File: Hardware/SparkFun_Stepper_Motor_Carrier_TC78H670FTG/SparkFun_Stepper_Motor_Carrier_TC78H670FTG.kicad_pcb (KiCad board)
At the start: 4 copper layers, 15.2 x 20.3 mm, 34 parts, among them J1 Conn_01x08, J2 Conn_01x08

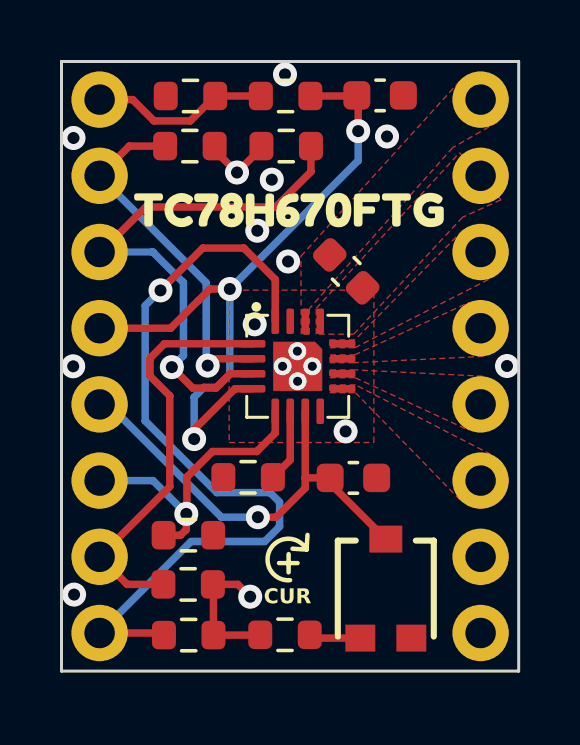
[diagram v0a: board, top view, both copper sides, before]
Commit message: version in bottom copper
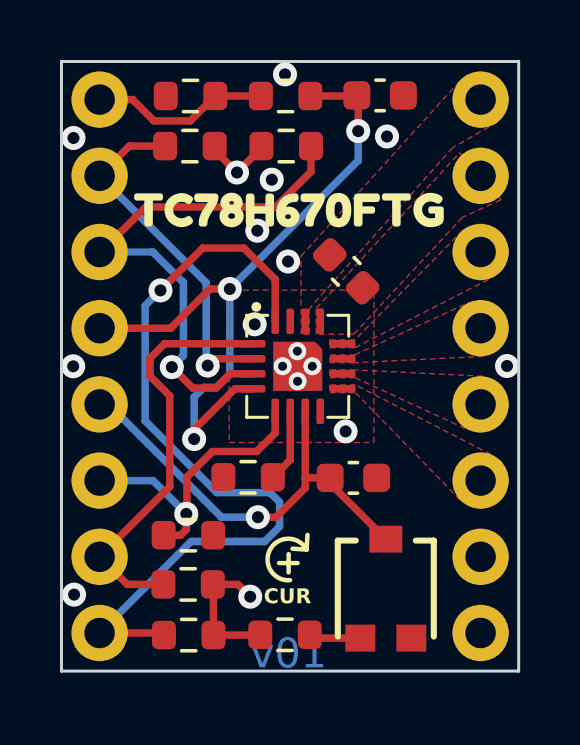
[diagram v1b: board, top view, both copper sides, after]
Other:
- board text added: "v01"
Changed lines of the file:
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@@
   (setup
     (stackup
-      (layer "F.SilkS" (type "Top Silk Screen"))
+      (layer "F.SilkS" (type "Top Silk Screen") (color "White"))
       (layer "F.Paste" (type "Top Solder Paste"))
-      (layer "F.Mask" (type "Top Solder Mask") (thickness 0.01))
+      (layer "F.Mask" (type "Top Solder Mask") (color "Red") (thickness 0.01))
       (layer "F.Cu" (type "copper") (thickness 0.035))
       (layer "dielectric 1" (type "prepreg") (thickness 0.1) (material "FR4") (epsilon_r 4.5) (loss_tangent 0.02))
@@
       (layer "dielectric 3" (type "prepreg") (thickness 0.1) (material "FR4") (epsilon_r 4.5) (loss_tangent 0.02))
       (layer "B.Cu" (type "copper") (thickness 0.035))
-      (layer "B.Mask" (type "Bottom Solder Mask") (thickness 0.01))
+      (layer "B.Mask" (type "Bottom Solder Mask") (color "Red") (thickness 0.01))
       (layer "B.Paste" (type "Bottom Solder Paste"))
-      (layer "B.SilkS" (type "Bottom Silk Screen"))
+      (layer "B.SilkS" (type "Bottom Silk Screen") (color "White"))
       (copper_finish "None")
       (dielectric_constraints no)
@@
   (gr_rect (start 134.62 93.98) (end 149.86 114.3)
     (stroke (width 0.1) (type default)) (fill none) (layer "Edge.Cuts"))
+  (gr_text "v01" (at 140.91 114.3) (layer "B.Cu")
+    (effects (font (size 1 1) (thickness 0.15)) (justify left bottom))
+  )
   (gr_text "CUR" (at 141.36 112.1) (layer "F.SilkS")
     (effects (font (size 0.5 0.5) (thickness 0.125) bold) (justify left bottom))
